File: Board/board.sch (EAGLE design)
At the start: 19 parts, among them IC1 L293D

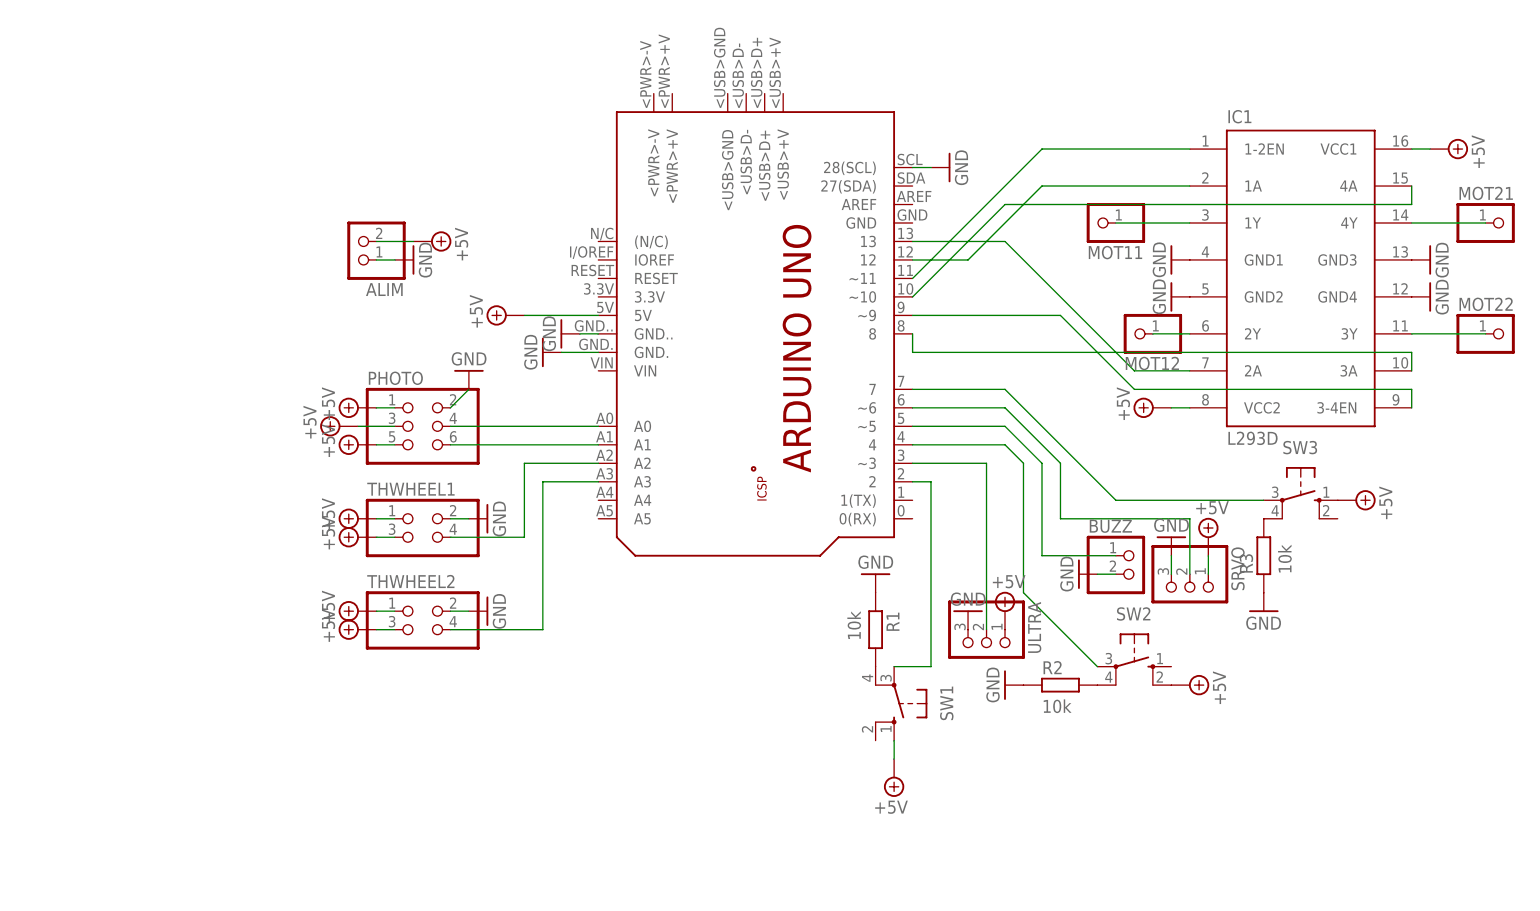
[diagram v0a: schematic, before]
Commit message: Updated boad
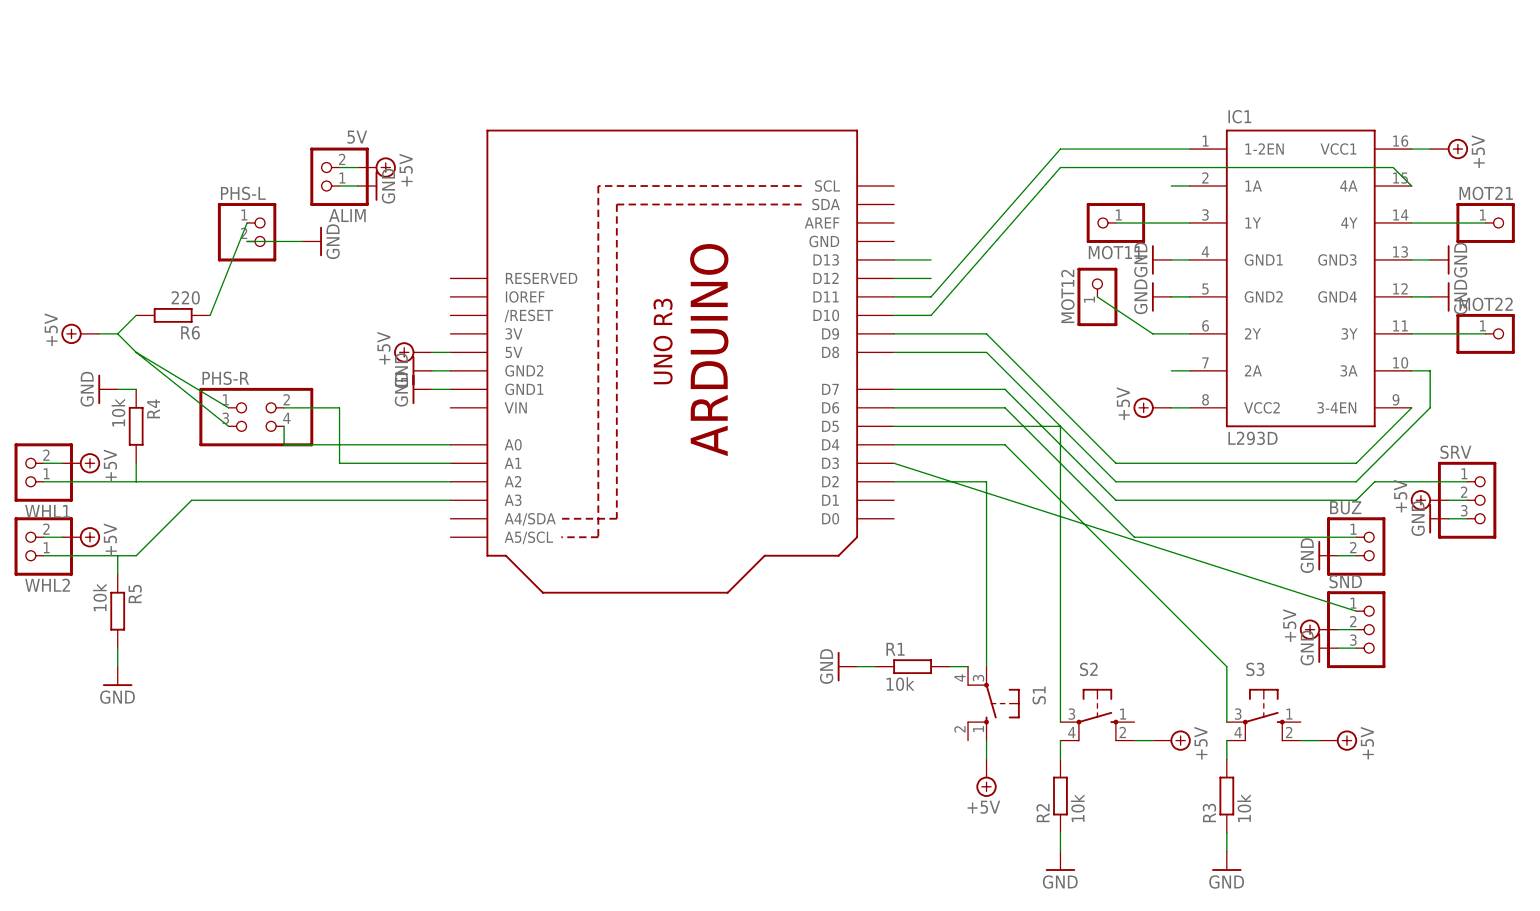
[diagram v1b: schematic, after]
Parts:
- removed BUZZ: (no value), pinhead:PINHD-1X2
- removed PCB1: ARDUINO_UNO, E14_Arduino_revB:ARDUINO_UNO
- removed PHOTO: (no value), pinhead:PINHD-2X3
- removed SRVO, ULTRA: (no value), pinhead:PINHD-1X3
- removed SW1, SW2, SW3: (no value), adafruit:40-XX
- removed THWHEEL1, THWHEEL2: (no value), pinhead:PINHD-2X2
- added BUZ, PHS-L, WHL1, WHL2: (no value), pinhead:PINHD-1X2
- added PHS-R: (no value), pinhead:PINHD-2X2
- added R4, R5: 10k, resistor:R-EU_R1206
- added R6: 220, resistor:R-EU_R1206
- added S1, S2, S3: (no value), switch-omron:10-XX
- added SND: (no value), pinhead:PINHD-1X3
- added SRV: (no value), pinhead:PINHD-1X3/90
- added U1: ARDUINOR3-BPLACE, adafruit:ARDUINOR3-BPLACE
- ALIM: value (none) -> 5V
- R1, R2, R3: device BaseApp:RESISTOR -> resistor:R-EU_R1206
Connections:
- removed net N$15: PCB1.~3, ULTRA.2
- removed net N$17: PCB1.7, SW3.P
- new net PIN12: IC1.1A, U1.D12
- new net PIN13: IC1.2A, U1.D13
- net +5V: now also PHS-R.1, PHS-R.3, R6.2, S1.S, S2.S1, S3.S1, SND.2, SRV.2, U1.5V, WHL1.2, WHL2.2; no longer PCB1.5V, PHOTO.1, PHOTO.3, PHOTO.5, SRVO.1, SW1.S, SW2.S1, SW3.S, THWHEEL1.1, THWHEEL1.3, THWHEEL2.1, THWHEEL2.3, ULTRA.1
- net GND: now also BUZ.2, PHS-L.2, R4.1, R5.2, SND.3, SRV.3, U1.GND1, U1.GND2; no longer BUZZ.2, PCB1.28(SCL), PCB1.GND., PCB1.GND.., SRVO.3, THWHEEL1.2, THWHEEL2.2, ULTRA.3
- net N$10: now also U1.D11; no longer PCB1.~11
- net N$11: now also R4.2, U1.A2, WHL1.1; no longer PCB1.A1, PHOTO.6
- net N$12: now also PHS-L.1, R6.1; no longer PCB1.A0, PHOTO.4
- net N$13: now also R5.1, U1.A3, WHL2.1; no longer PHOTO.2
- net N$14: now also SRV.1, U1.D7; no longer PCB1.~6, SRVO.2
- net N$16: now also BUZ.1, U1.D6; no longer BUZZ.1, PCB1.~5
- net N$18: now also R2.2, S2.P1; no longer R3.2, SW3.P1
- net N$19: now also S3.P, U1.D4; no longer PCB1.4, SW2.P
- net N$20: now also R3.2, S3.P1; no longer R2.2, SW2.P1
- net N$21: now also S1.P1; no longer SW1.P1
- net N$22: now also SND.1, U1.D3; no longer PCB1.A2, THWHEEL1.4
- net N$23: now also S2.P, U1.D5; no longer PCB1.A3, THWHEEL2.4
- net N$24: now also S1.P, U1.D2; no longer PCB1.2, SW1.P
- net N$5: now also PHS-R.2, U1.A1; no longer IC1.1A, PCB1.12
- net N$6: now also PHS-R.4, U1.A0; no longer IC1.2A, PCB1.13
- net N$7: now also U1.D10; no longer PCB1.~10
- net N$8: now also U1.D9; no longer PCB1.~9
- net N$9: now also U1.D8; no longer PCB1.8
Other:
- moved on the sheet: ALIM, MOT12, R1, R2, R3
